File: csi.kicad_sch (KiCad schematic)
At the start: 65 parts, among them J1 200528-0150, J12 200528-0150, J6 200528-0150, J9 200528-0150, U24 AP22615A, U25 AP22615A, U26 PI4MSD5V9548AZDEX, U3 AP22615A, U31 NTS0102, U32 NTS0102, U7 AP22615A

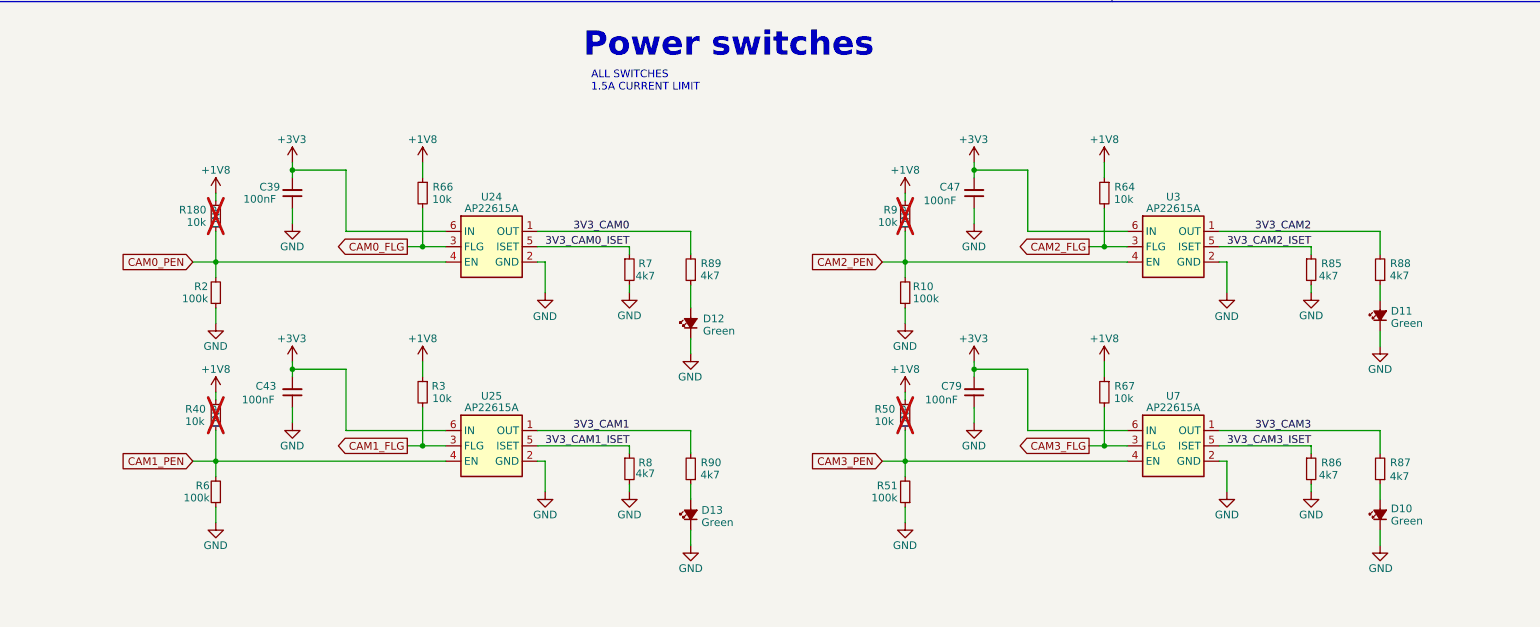
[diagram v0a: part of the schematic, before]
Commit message: v2.0 Schematic updates
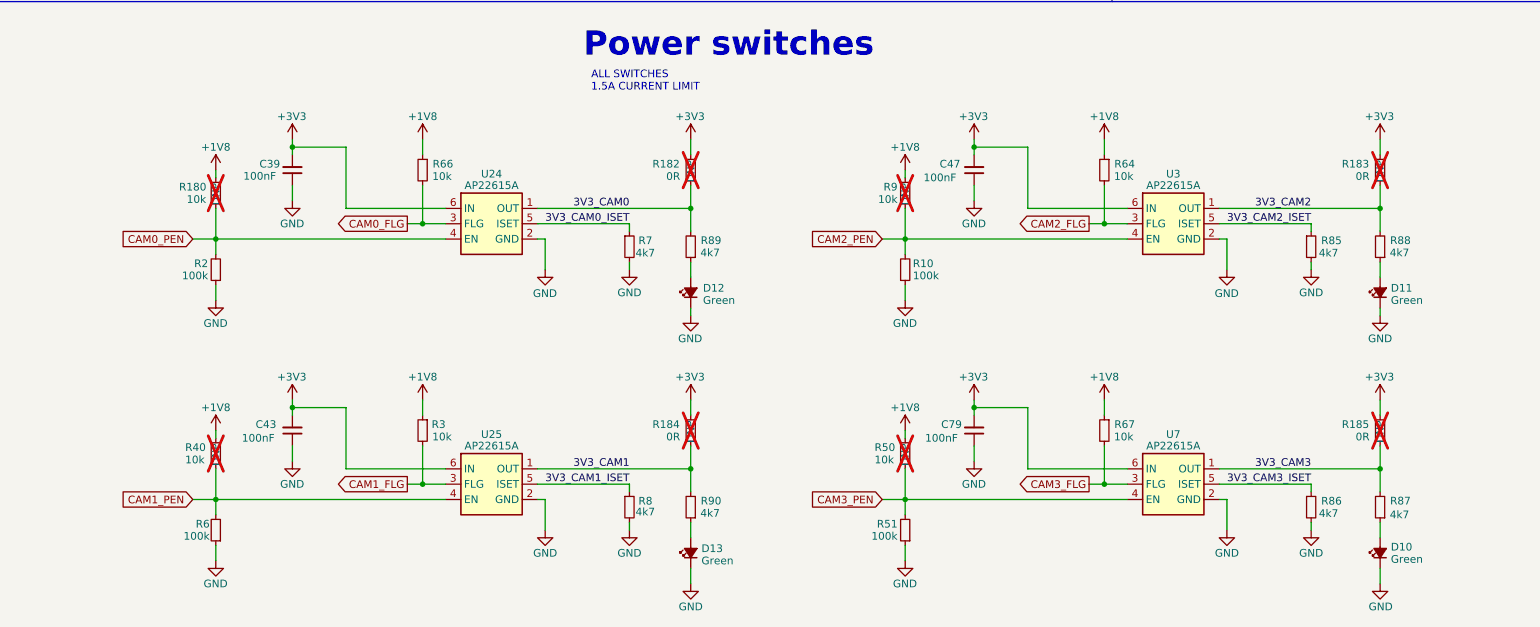
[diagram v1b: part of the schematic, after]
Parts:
- added R182, R183, R184, R185: 0R, Resistor_SMD:R_0603_1608Metric, symbol Device:R_Small
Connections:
- net +3V3: now also R182.1, R183.1, R184.1, R185.1
- net 3V3_CAM0: now also R182.2
- net 3V3_CAM1: now also R184.2
- net 3V3_CAM2: now also R183.2
- net 3V3_CAM3: now also R185.2
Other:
- company: Argus-1 Cubesat -> Carnegie Mellon University
- title: Jetson Carrier Board -> Argus Carrierboard
- moved on the sheet: C39, C43, C47, C79, D10, D11, D12, D13, R10, R180, R2, R3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
